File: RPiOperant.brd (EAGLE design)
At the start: 120 x 94 mm, 63 parts, among them IC1 74LS14N, IC2 74LS14N, J2 POWER_JACK, X1 2516-, X3 2550-

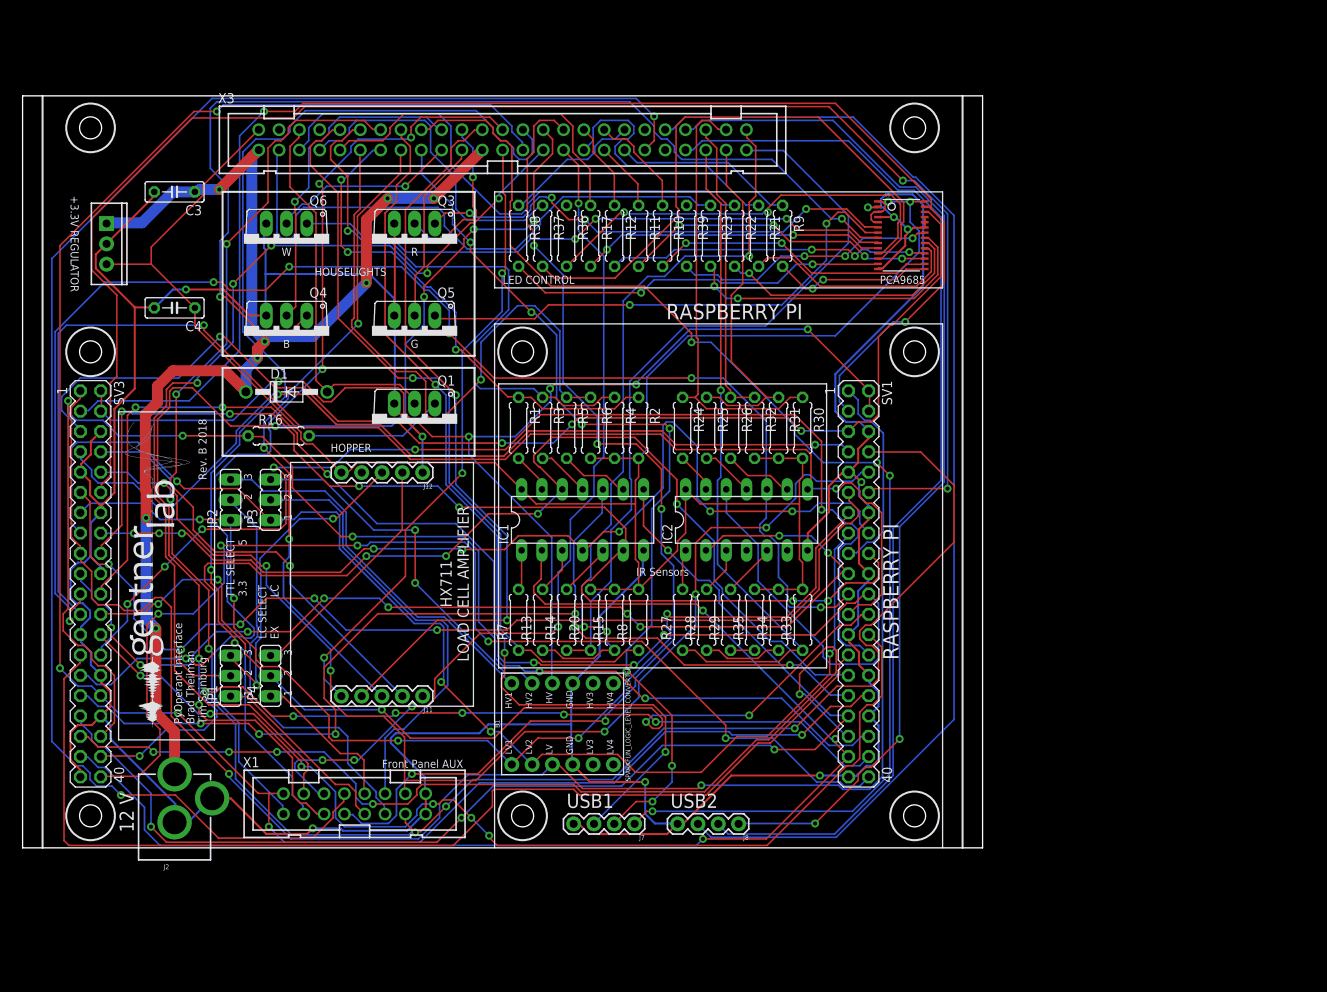
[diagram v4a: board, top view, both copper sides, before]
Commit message: rev_b layout
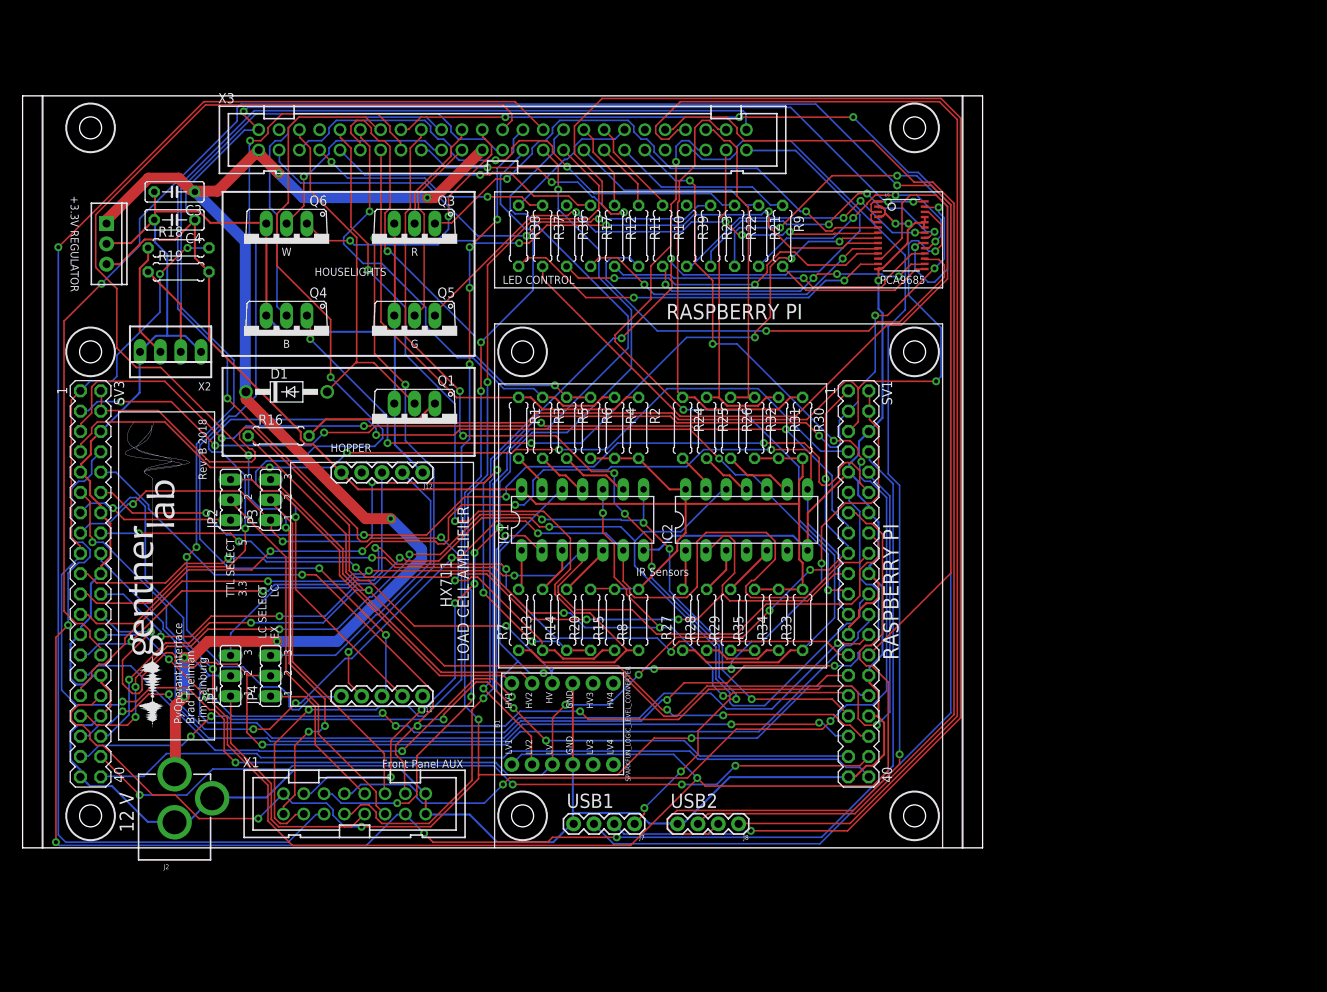
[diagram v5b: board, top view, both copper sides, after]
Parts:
- added R18, R19: 330, resistor:0207/7
- added X2: 22-23-2041, con-molex:22-23-2041
- moved C4 11.0 mm to (19.0, 78.5)
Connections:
- new net N$25: R19.1, X2.2
- new net N$31: R18.1, X2.3
- net +3V3: now also R19.2
- net GND: now also X2.1, X2.4
- net RPI_3.3V: now also R18.2
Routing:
- net USB1_D-: track 112.3 -> 218.9 mm, vias 7 -> 4
- net ID_SC: track 145.9 -> 234.8 mm, vias 6 -> 2
- net PCM_CLK: track 199.1 -> 111.9 mm, vias 2 -> 4
- net IR_1: track 93.4 -> 173.0 mm
- net GPIO27: track 139.4 -> 217.8 mm, vias 5 -> 3
- net USB1_D+: track 116.9 -> 189.9 mm
- net LOADCELLE+: track 78.7 -> 131.6 mm, vias 3 -> 2
- net IR_5_GPIO: track 171.9 -> 126.3 mm, vias 2 -> 4
- net GND: track 488.8 -> 443.3 mm, vias 9 -> 3
- net PCM_DOUT: track 142.9 -> 99.1 mm, vias 5 -> 0
- net IR_4_GPIO: track 177.4 -> 134.2 mm, vias 6 -> 4
- net IR_3_GPIO: track 183.5 -> 140.6 mm, vias 6 -> 4
- net USB1_VBUS: track 158.5 -> 118.8 mm, vias 4 -> 8
- net SDA: track 177.9 -> 139.1 mm, vias 2 -> 7
- net AUX2: track 243.6 -> 207.8 mm, vias 5 -> 6
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
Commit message: revb
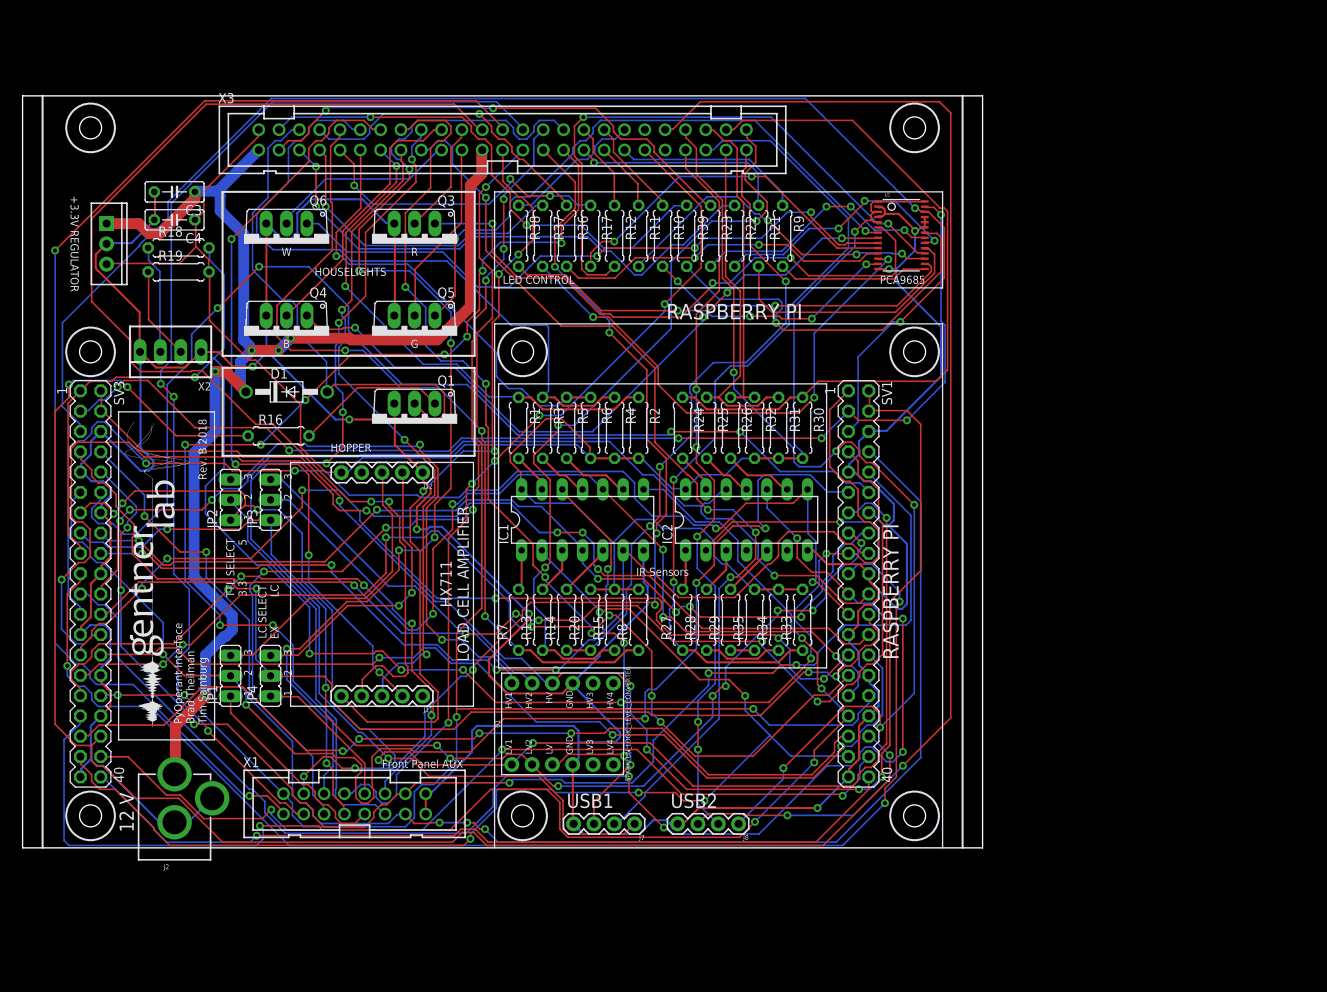
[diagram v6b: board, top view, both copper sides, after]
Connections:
- removed net CENTNER_LED: R36.1
- removed net RGB_CUE_B\: X3.4
- net CENTER_LED: now also R36.1
- net RGB_CUE_B: now also X3.4
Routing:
- net ID_SC: track 234.8 -> 118.8 mm, vias 2 -> 3
- net USB1_D-: track 218.9 -> 118.6 mm
- net IR_1: track 173.0 -> 96.0 mm
- net USB1_D+: track 189.9 -> 113.8 mm, vias 3 -> 6
- net IR_6_GPIO: track 116.3 -> 190.8 mm
- net GND: track 443.3 -> 510.3 mm, vias 3 -> 7
- net RGB_CUE_B: track 0.00 -> 64.3 mm, vias 0 -> 2
- net AUX5: track 178.1 -> 116.0 mm, vias 1 -> 6
- net LOADCELLE-: track 90.4 -> 147.3 mm, vias 4 -> 2
- net HOPPER_TRIG_GPIO: track 139.7 -> 193.0 mm, vias 5 -> 3
- net AUX8: track 160.2 -> 109.7 mm, vias 6 -> 5
- net USB2_D-: track 140.5 -> 91.8 mm, vias 1 -> 5
- net GPIO4: track 108.2 -> 152.0 mm, vias 3 -> 6
- net CENTER_PECK_GPIO: track 130.1 -> 173.3 mm, vias 8 -> 5
- net IR_4_GPIO: track 134.2 -> 176.7 mm, vias 4 -> 5
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
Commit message: rev_c v1
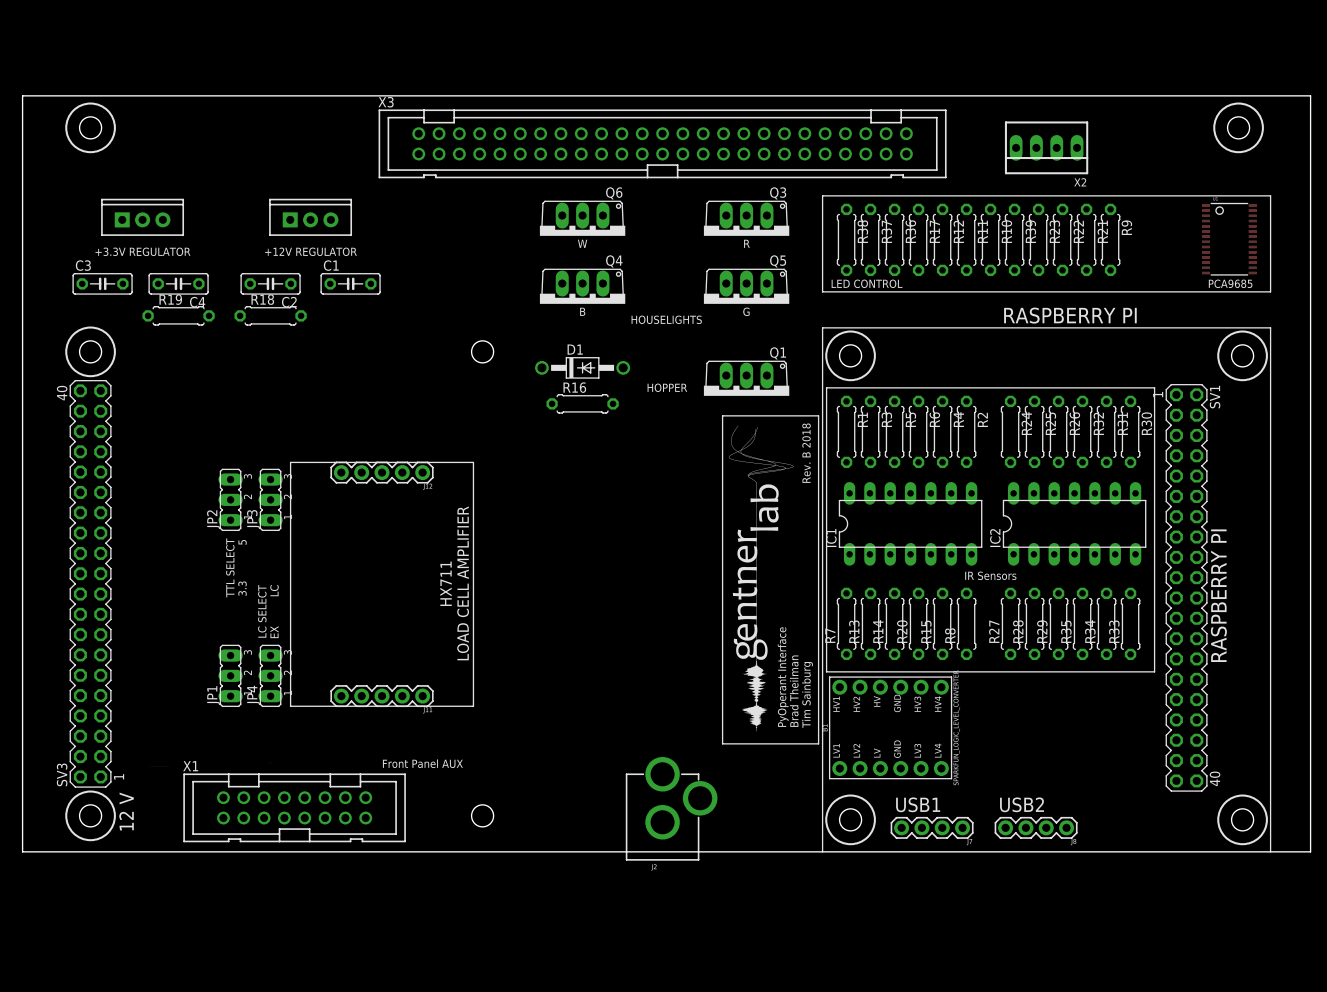
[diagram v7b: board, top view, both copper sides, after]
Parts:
- added C1: 100nF, adafruit:C050-025X075
- added C2: 10uF, adafruit:C050-025X075
- added U3: (no value), SparkFun-IC-Power:TO220-IGO
- moved X2 112.4 mm to (128.0, 87.5)
- moved J2 61.0 mm to (80.0, -4.50)
- moved Q5 41.7 mm to (90.5, 68.0)
- moved Q1 41.6 mm to (90.5, 56.5)
- moved Q3 41.5 mm to (90.5, 76.5)
- moved B1 41.0 mm to (108.5, 15.0)
- moved IC1 41.0 mm to (111.0, 40.5)
- moved IC2 41.0 mm to (131.5, 40.5)
- moved J7 41.0 mm to (117.5, 2.50)
- moved J8 41.0 mm to (130.5, 2.50)
- moved R1 41.0 mm to (103.0, 52.0)
- moved R10 41.0 mm to (121.0, 76.0)
- moved R11 41.0 mm to (118.0, 76.0)
- moved R12 41.0 mm to (115.0, 76.0)
- moved R13 41.0 mm to (106.0, 28.0)
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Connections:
- new net 24V: C1.1, C3.1, J2.PWR, U2.IN, U3.IN, X3.1
- net 12V: now also C2.1, U3.OUT; no longer C3.1, J2.PWR, U2.IN, X3.1
- net GND: now also C1.2, C2.2, U3.GND
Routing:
- net GND: track 510.3 -> 0.00 mm, vias 7 -> 0
- net +3V3: track 251.2 -> 0.00 mm, vias 1 -> 0
- net RPI_3.3V: track 231.9 -> 0.00 mm, vias 8 -> 0
- net AUX2: track 194.3 -> 0.00 mm, vias 5 -> 0
- net HOPPER_TRIG_GPIO: track 193.0 -> 0.00 mm, vias 3 -> 0
- net IR_6_GPIO: track 190.8 -> 0.00 mm, vias 4 -> 0
- net TXD: track 182.7 -> 0.00 mm, vias 5 -> 0
- net RPI_5V: track 181.7 -> 0.00 mm, vias 5 -> 0
- net GPIO27: track 177.9 -> 0.00 mm, vias 6 -> 0
- net IR_4_GPIO: track 176.7 -> 0.00 mm, vias 5 -> 0
- net SCL: track 175.3 -> 0.00 mm, vias 2 -> 0
- net CENTER_PECK_GPIO: track 173.3 -> 0.00 mm, vias 5 -> 0
- net RXD: track 169.1 -> 0.00 mm, vias 6 -> 0
- net 12V: track 163.3 -> 0.00 mm, vias 5 -> 0
- net GPIO17: track 159.0 -> 0.00 mm, vias 5 -> 0
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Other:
- board size 120 x 94 mm -> 161 x 94.5 mm
- board text added: "+12V REGULATOR"
